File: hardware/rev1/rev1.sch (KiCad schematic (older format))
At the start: 43 parts, among them J1 Conn_01x09_Female, J2 RFM9X_header, J3 Conn_01x03_Male, Q1 Q_PNP_BCE, U1 BNO055, U2 MPL3115A2, U3 Teensy3.6, U4 BMI088, U5 ADXL345BCCZ, Y1 Crystal_32kHz768

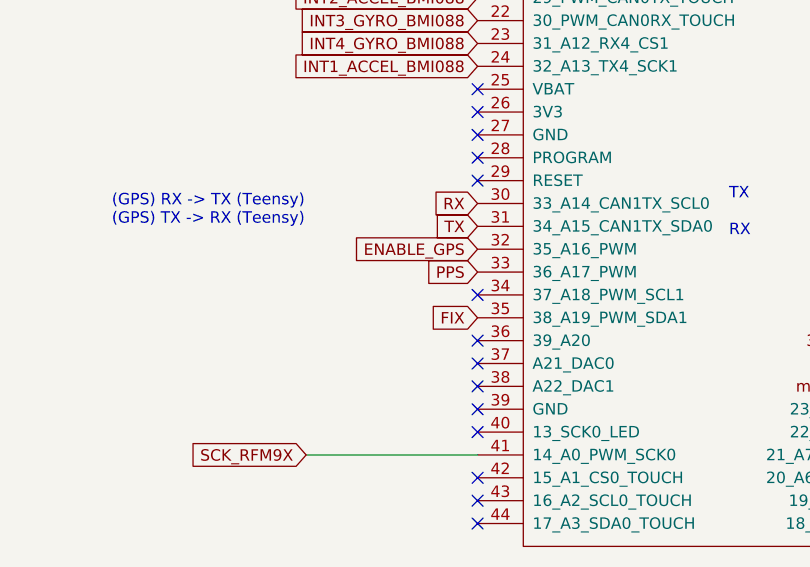
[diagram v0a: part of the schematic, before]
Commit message: rearrange GPS
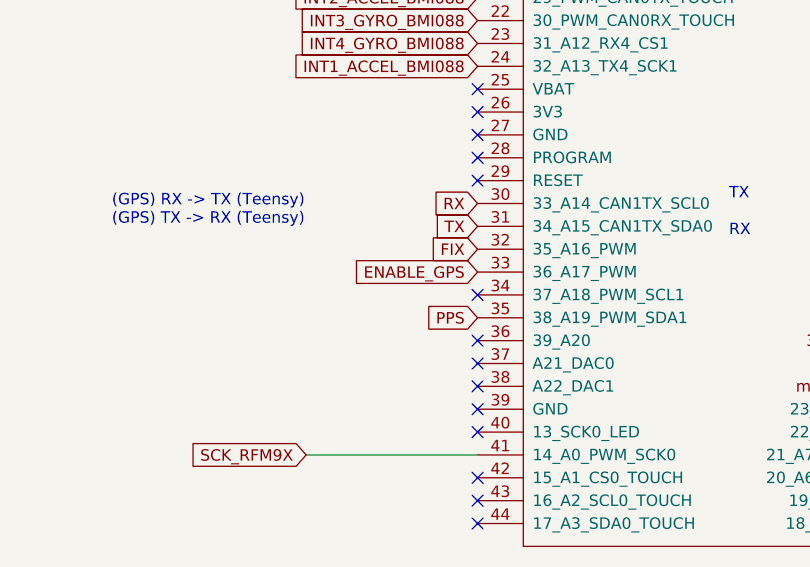
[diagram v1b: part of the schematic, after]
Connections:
- net ENABLE_GPS: now also U3.33 (36_A17_PWM); no longer U3.32 (35_A16_PWM)
- net FIX: now also U3.32 (35_A16_PWM); no longer U3.35 (38_A19_PWM_SDA1)
- net PPS: now also U3.35 (38_A19_PWM_SDA1); no longer U3.33 (36_A17_PWM)
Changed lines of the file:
@@
 Text GLabel 27400 5800 0    50   Input ~ 0
 TX
-Text GLabel 27400 6200 0    50   Input ~ 0
+Text GLabel 27400 5900 0    50   Input ~ 0
 FIX
-Text GLabel 27400 5900 0    50   Input ~ 0
+Text GLabel 27400 6000 0    50   Input ~ 0
 ENABLE_GPS
 NoConn ~ 29700 3400
@@
 Wire Wire Line
 	13700 16450 13700 16600
-Text GLabel 27400 6000 0    50   Input ~ 0
+Text GLabel 27400 6200 0    50   Input ~ 0
 PPS
 $Comp
